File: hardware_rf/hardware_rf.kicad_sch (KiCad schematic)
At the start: 63 parts, among them IC1 CC1125RHBR, IC2 BALF-SPI2-02D3, IC3 4259-63, IC4 4259-63, J1 Conn_Coaxial, J2 Conn_01x03_Socket, SW1 SW_Push, U1 RP2350A-QFN60, U2 W25Q128JVS, U3 GSQ5111, U4 SK5129, Y1 Crystal_GND24, Y2 Crystal_GND24

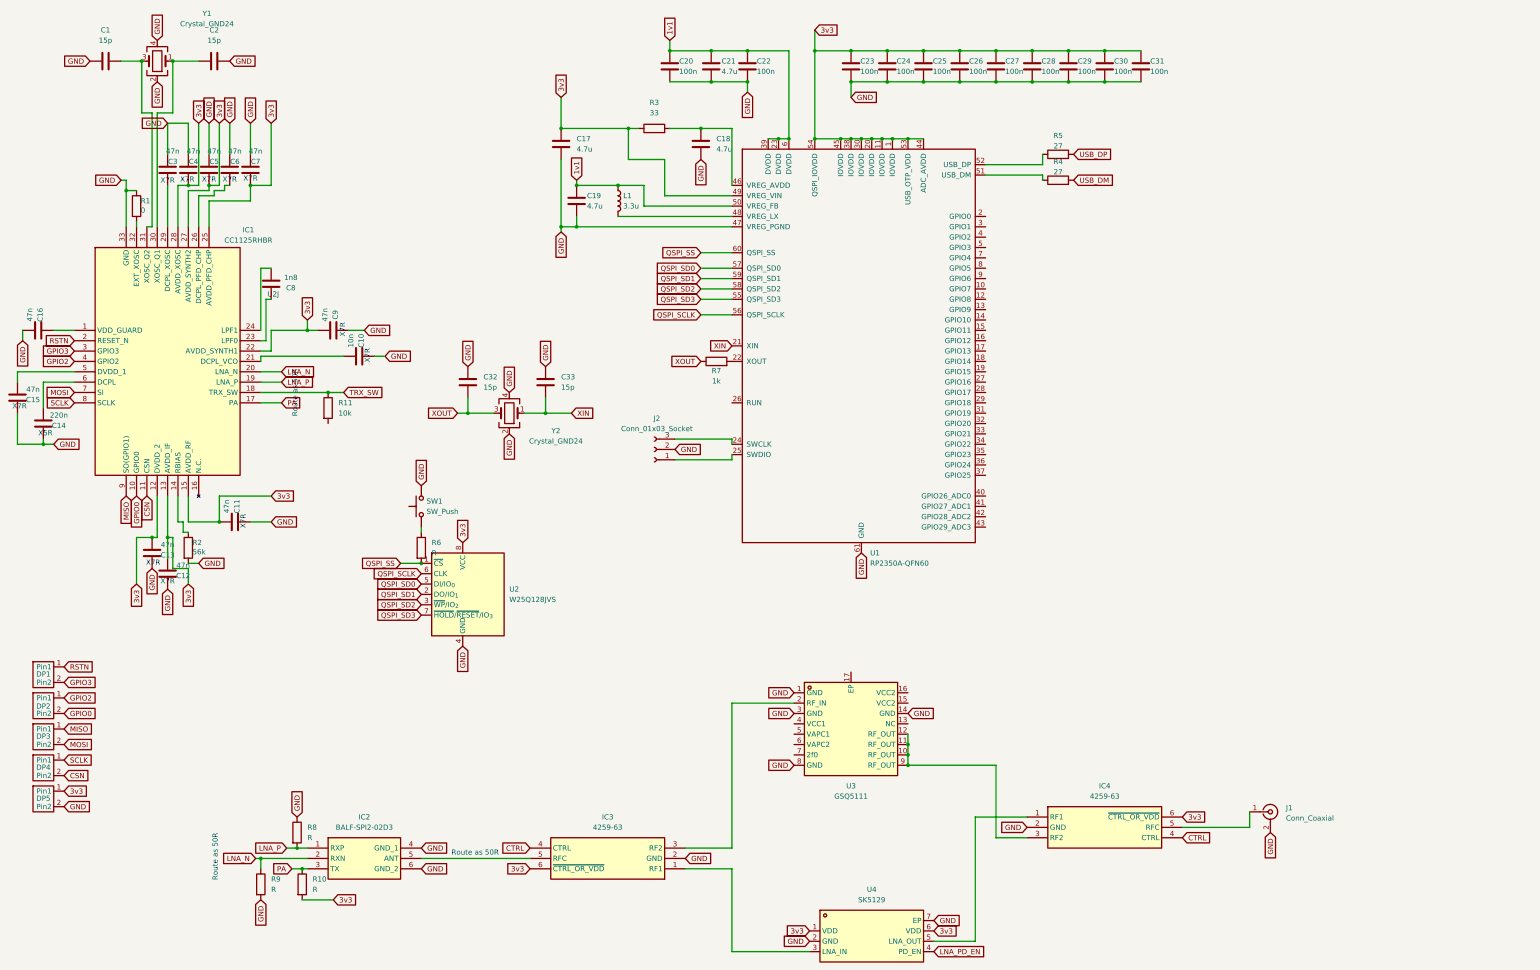
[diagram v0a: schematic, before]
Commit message: Schematic Done
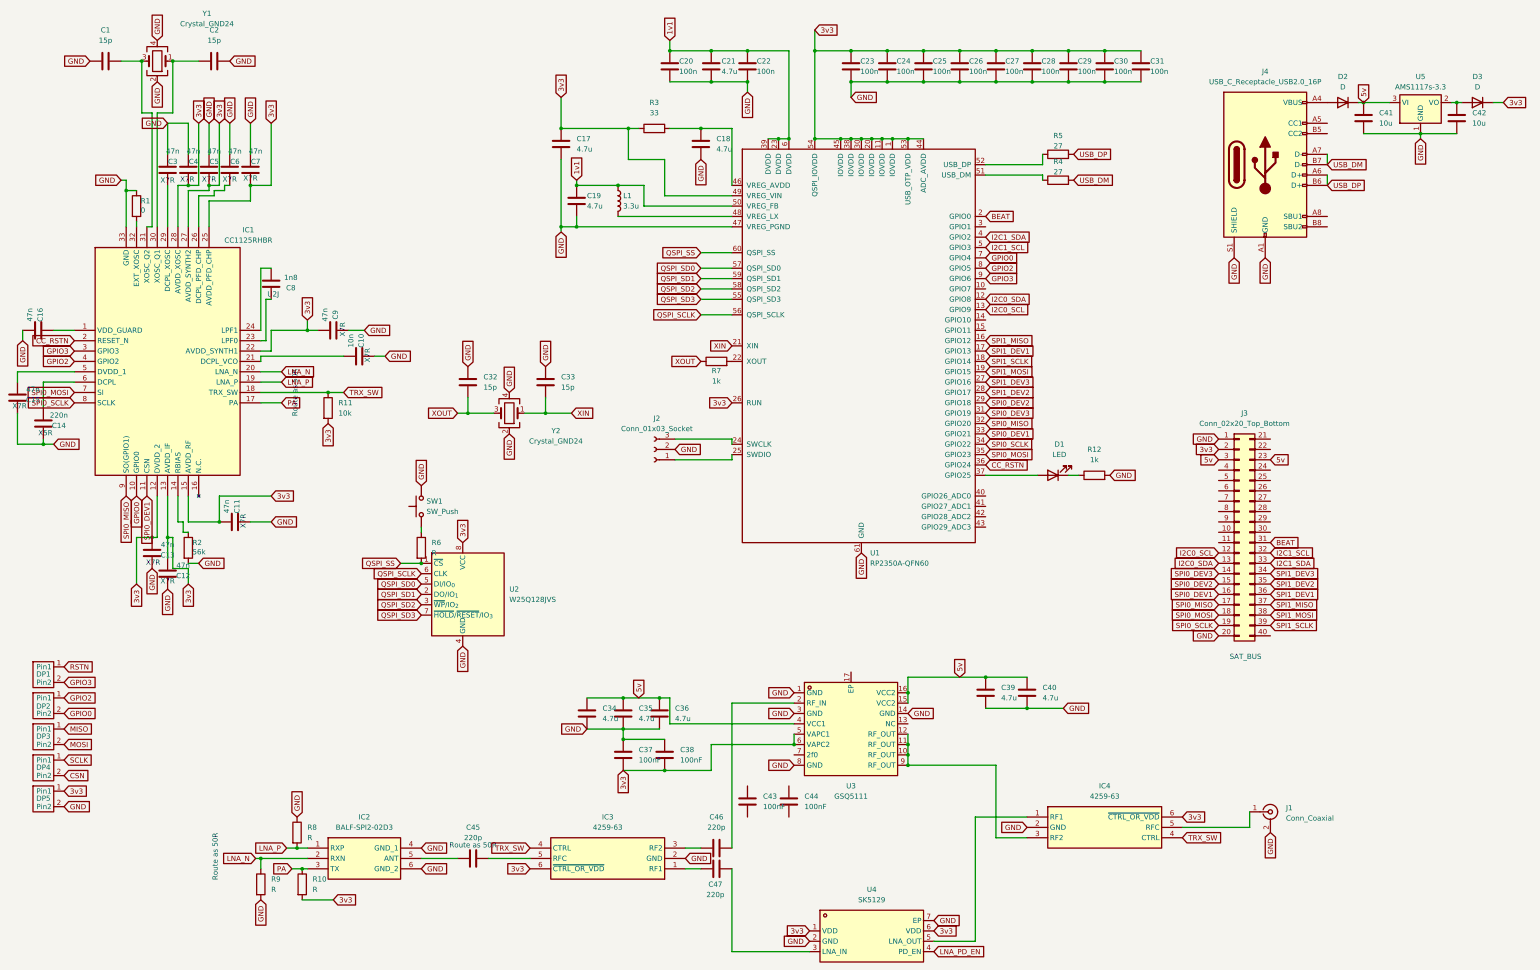
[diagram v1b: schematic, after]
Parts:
- added C34, C35, C36, C39, C40: 4.7u, symbol Device:C
- added C37, C38, C43, C44: 100nF, symbol Device:C
- added C41, C42: 10u, symbol Device:C
- added C45, C46, C47: 220p, symbol Device:C
- added D1: LED, symbol Device:LED
- added D2, D3: D, symbol Device:D
- added J3: Conn_02x20_Top_Bottom, symbol Connector_Generic:Conn_02x20_Top_Bottom
- added J4: USB_C_Receptacle_USB2.0_16P, symbol Connector:USB_C_Receptacle_USB2.0_16P
- added R12: 1k, symbol Device:R
- added U5: AMS1117s-3.3, Package_TO_SOT_SMD:SOT-89-3, symbol Regulator_Linear:AMS1117-3.3
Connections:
- net CTRL is gone; now on net TRX_SW: IC3.4 (CTRL), IC4.4 (CTRL)
- net 3v3: now also R11.2, U1.26 (RUN), U3.5 (VAPC1), U3.6 (VAPC2), C37.2, C38.2, D3.1 (K), J3.2 (Pin_2)
- net CSN: no longer IC1.11 (CSN)
- net GND: now also C34.2, C35.2, C36.2, C37.1, C38.1, C39.2, C40.2, C41.2, C42.2, J3.1 (Pin_1), J3.20 (Pin_20), J4.A1 (GND), J4.A12 (GND), J4.B1 (GND), J4.B12 (GND), J4.S1 (SHIELD), R12.2, U5.1 (GND)
- net GPIO0: now also U1.7 (GPIO4)
- net GPIO2: now also U1.8 (GPIO5)
- net GPIO3: now also U1.9 (GPIO6)
- net MISO: no longer IC1.9 (SO(GPIO1))
- net MOSI: no longer IC1.7 (SI)
- net RSTN: no longer IC1.2 (RESET_N)
- net SCLK: no longer IC1.8 (SCLK)
- net USB_DM: now also J4.A7 (D-), J4.B7 (D-)
- net USB_DP: now also J4.A6 (D+), J4.B6 (D+)
- net 5v: now reaches U3.15 (VCC2)
- net 5v: now also U3.16 (VCC2), U3.4 (VCC1), C34.1, C35.1, C36.1, C39.1, C40.1, C41.1, D2.1 (K), J3.23 (Pin_23), J3.3 (Pin_3), U5.3 (VI)
- net at IC3.3 (RF2): now also C46.1; no longer U3.2 (RF_IN)
- net at IC3.1 (RF1): now also C47.1; no longer U4.3 (LNA_IN)
- net I2C0_SDA: now reaches U1.12 (GPIO8)
- net I2C0_SDA: now also J3.13 (Pin_13)
- net I2C0_SCL: now reaches U1.13 (GPIO9)
- net I2C0_SCL: now also J3.12 (Pin_12)
- net SPI1_MISO: now reaches U1.16 (GPIO12)
- net SPI1_MISO: now also J3.37 (Pin_37)
- net SPI1_DEV1: now reaches U1.17 (GPIO13)
- net SPI1_DEV1: now also J3.36 (Pin_36)
- net SPI1_SCLK: now reaches U1.18 (GPIO14)
- net SPI1_SCLK: now also J3.39 (Pin_39)
- net SPI1_MOSI: now reaches U1.19 (GPIO15)
- net SPI1_MOSI: now also J3.38 (Pin_38)
- net BEAT: now reaches U1.2 (GPIO0)
- net BEAT: now also J3.31 (Pin_31)
- net SPI1_DEV3: now reaches U1.27 (GPIO16)
- net SPI1_DEV3: now also J3.34 (Pin_34)
- net SPI1_DEV2: now reaches U1.28 (GPIO17)
- net SPI1_DEV2: now also J3.35 (Pin_35)
- net SPI0_DEV2: now reaches U1.29 (GPIO18)
- net SPI0_DEV2: now also J3.15 (Pin_15)
- net SPI0_DEV3: now reaches U1.31 (GPIO19)
- net SPI0_DEV3: now also J3.14 (Pin_14)
- net SPI0_MISO: now reaches U1.32 (GPIO20)
- net SPI0_MISO: now also IC1.9 (SO(GPIO1)), J3.17 (Pin_17)
- net SPI0_DEV1: now reaches U1.33 (GPIO21)
- net SPI0_DEV1: now also IC1.11 (CSN), J3.16 (Pin_16)
- net SPI0_SCLK: now reaches U1.34 (GPIO22)
- net SPI0_SCLK: now also IC1.8 (SCLK), J3.19 (Pin_19)
- net SPI0_MOSI: now reaches U1.35 (GPIO23)
- net SPI0_MOSI: now also IC1.7 (SI), J3.18 (Pin_18)
- net CC_RSTN: now reaches U1.36 (GPIO24)
- net CC_RSTN: now also IC1.2 (RESET_N)
- net at U1.37 (GPIO25): now also D1.2 (A)
- net I2C1_SDA: now reaches U1.4 (GPIO2)
- net I2C1_SDA: now also J3.33 (Pin_33)
- net I2C1_SCL: now reaches U1.5 (GPIO3)
- net I2C1_SCL: now also J3.32 (Pin_32)
- net at IC2.5 (ANT): now also C45.1; no longer IC3.5 (RFC)
- new net: D2.2 (A), J4.A4 (VBUS), J4.A9 (VBUS), J4.B4 (VBUS), J4.B9 (VBUS)
- new net: C47.2, U4.3 (LNA_IN)
- new net: C42.1, D3.2 (A), U5.2 (VO)
- new net: C46.2, U3.2 (RF_IN)
- new net: C45.2, IC3.5 (RFC)
- new net: D1.1 (K), R12.1
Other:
- note added: "SAT_BUS"

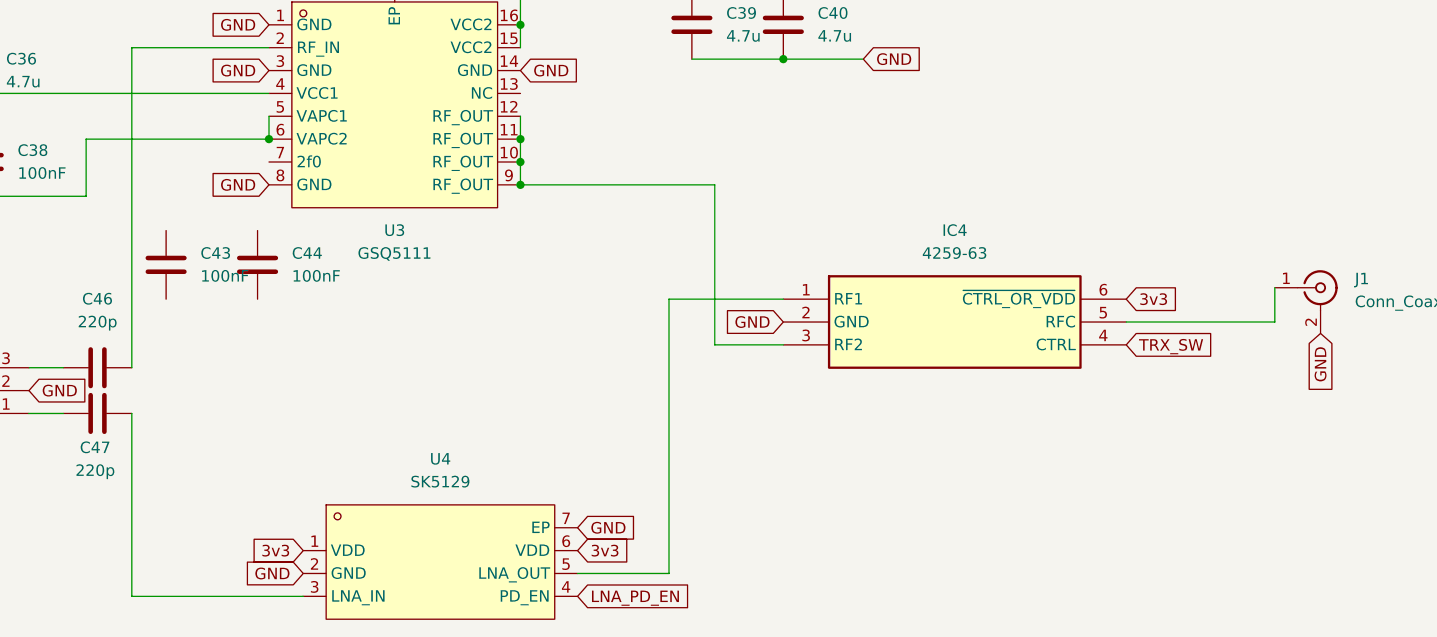
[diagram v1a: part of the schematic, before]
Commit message: assignment
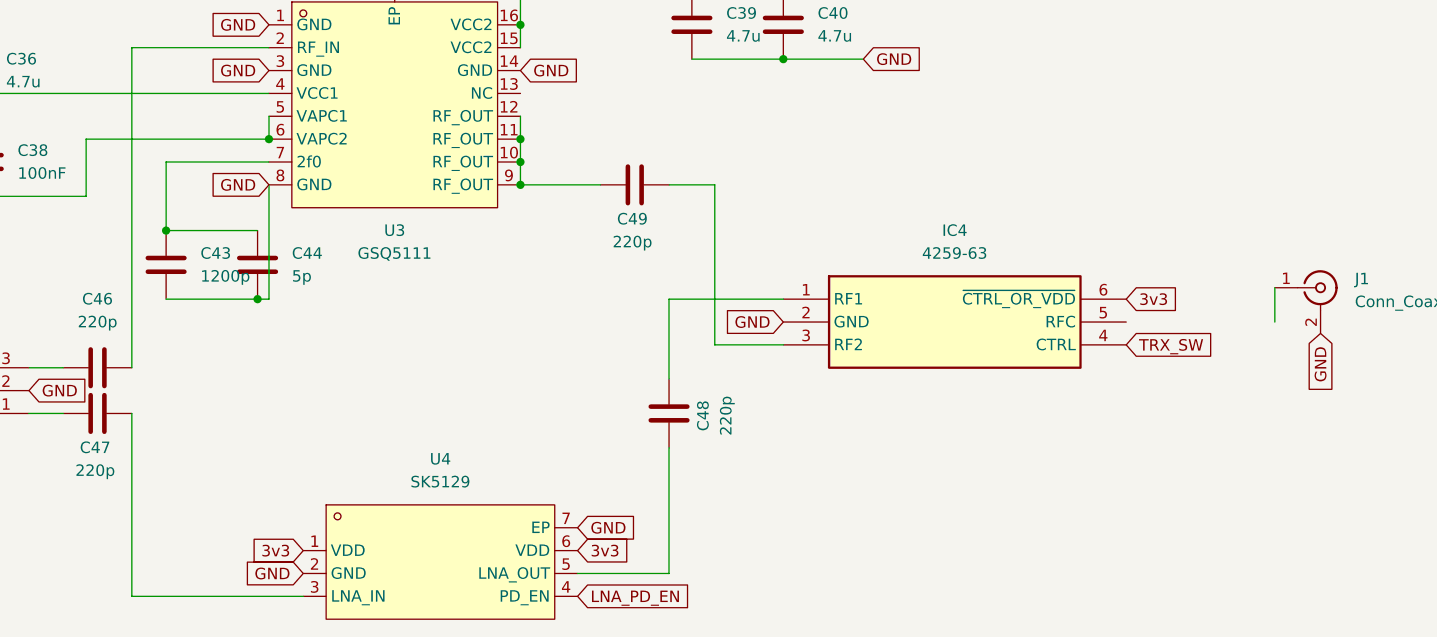
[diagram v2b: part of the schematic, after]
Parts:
- added C48, C49: 220p, Capacitor_SMD:C_0402_1005Metric, symbol Device:C
- C1, C10, C11, C12, C13, C14, C15, C16, C17, C18, C19, C2, C20, C21, C22, C23, C24, C25, C26, C27, C28, C29, C3, C30, C31, C32, C33, C34, C35, C36, C37, C38, C39, C4, C40, C45, C46, C47, C5, C6, C7, C8, C9: footprint (none) -> Capacitor_SMD:C_0402_1005Metric
- C41, C42: footprint (none) -> Capacitor_SMD:C_0805_2012Metric
- C43: value 100nF -> 1200p; footprint (none) -> Capacitor_SMD:C_0402_1005Metric
- C44: value 100nF -> 5p; footprint (none) -> Capacitor_SMD:C_0402_1005Metric
- J2: footprint (none) -> Connector_PinHeader_2.54mm:PinHeader_1x03_P2.54mm_Vertical
- J3: footprint (none) -> Connector_PinHeader_2.54mm:PinHeader_2x20_P2.54mm_Vertical
- J4: footprint (none) -> Connector_USB:USB_C_Receptacle_XKB_U262-16XN-4BVC11
- Y1, Y2: footprint (none) -> Crystal:Crystal_SMD_3225-4Pin_3.2x2.5mm
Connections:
- net GND: now also C43.2, C44.2
- net at C44.1: now also C43.1, U3.7 (2f0)
- net at U3.10 (RF_OUT), U3.11 (RF_OUT), U3.12 (RF_OUT)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: now also C49.1; no longer IC4.3 (RF2)
- net at J1.1 (In): no longer IC4.5 (RFC)
- net at U4.5 (LNA_OUT): now also C48.1; no longer IC4.1 (RF1)
- new net: C49.2, IC4.3 (RF2)
- new net: C48.2, IC4.1 (RF1)
